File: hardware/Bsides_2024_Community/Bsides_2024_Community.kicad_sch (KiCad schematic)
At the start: 41 parts, among them J1 Conn_02x03_Odd_Even, J2 Battery, J3 Battery, J4 OLED, J5 Conn_01x05, J6 Conn_01x05, P1 USB_C_Plug_USB2.0, Q1 DMG3415U-7, SW1 ON, SW2 RESET, SW3 BOOT, SW4 RESET, SW6 RESET, U1 ESP32-C6-WROOM-1U-N4, U2 AP2112K-3.3

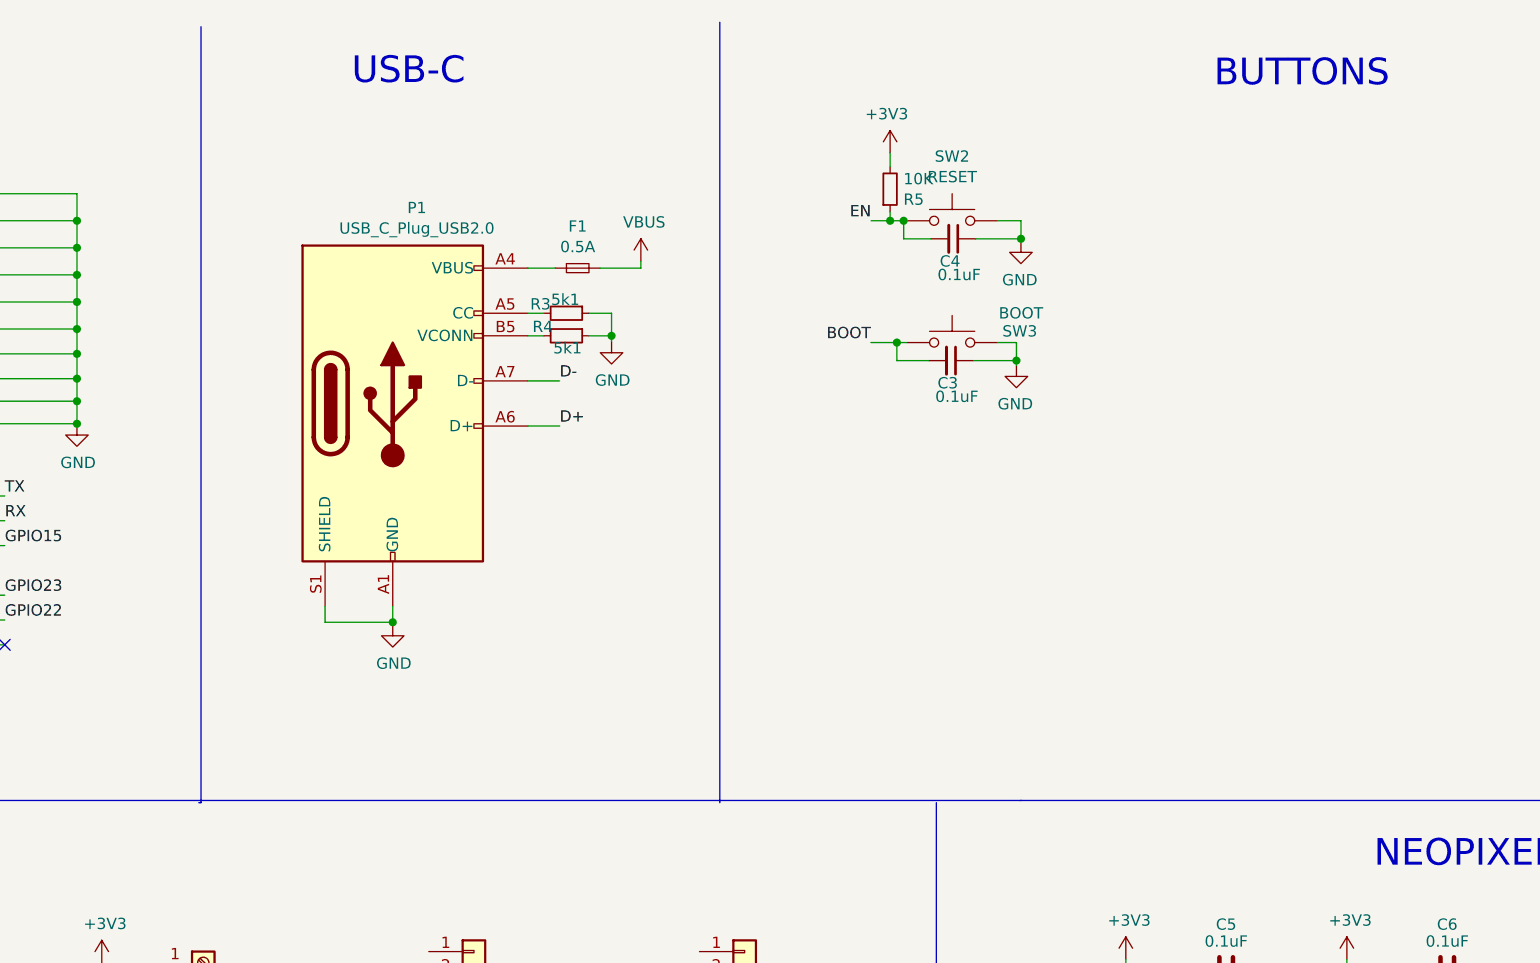
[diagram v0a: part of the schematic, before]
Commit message: feat(Hw): Update PCB
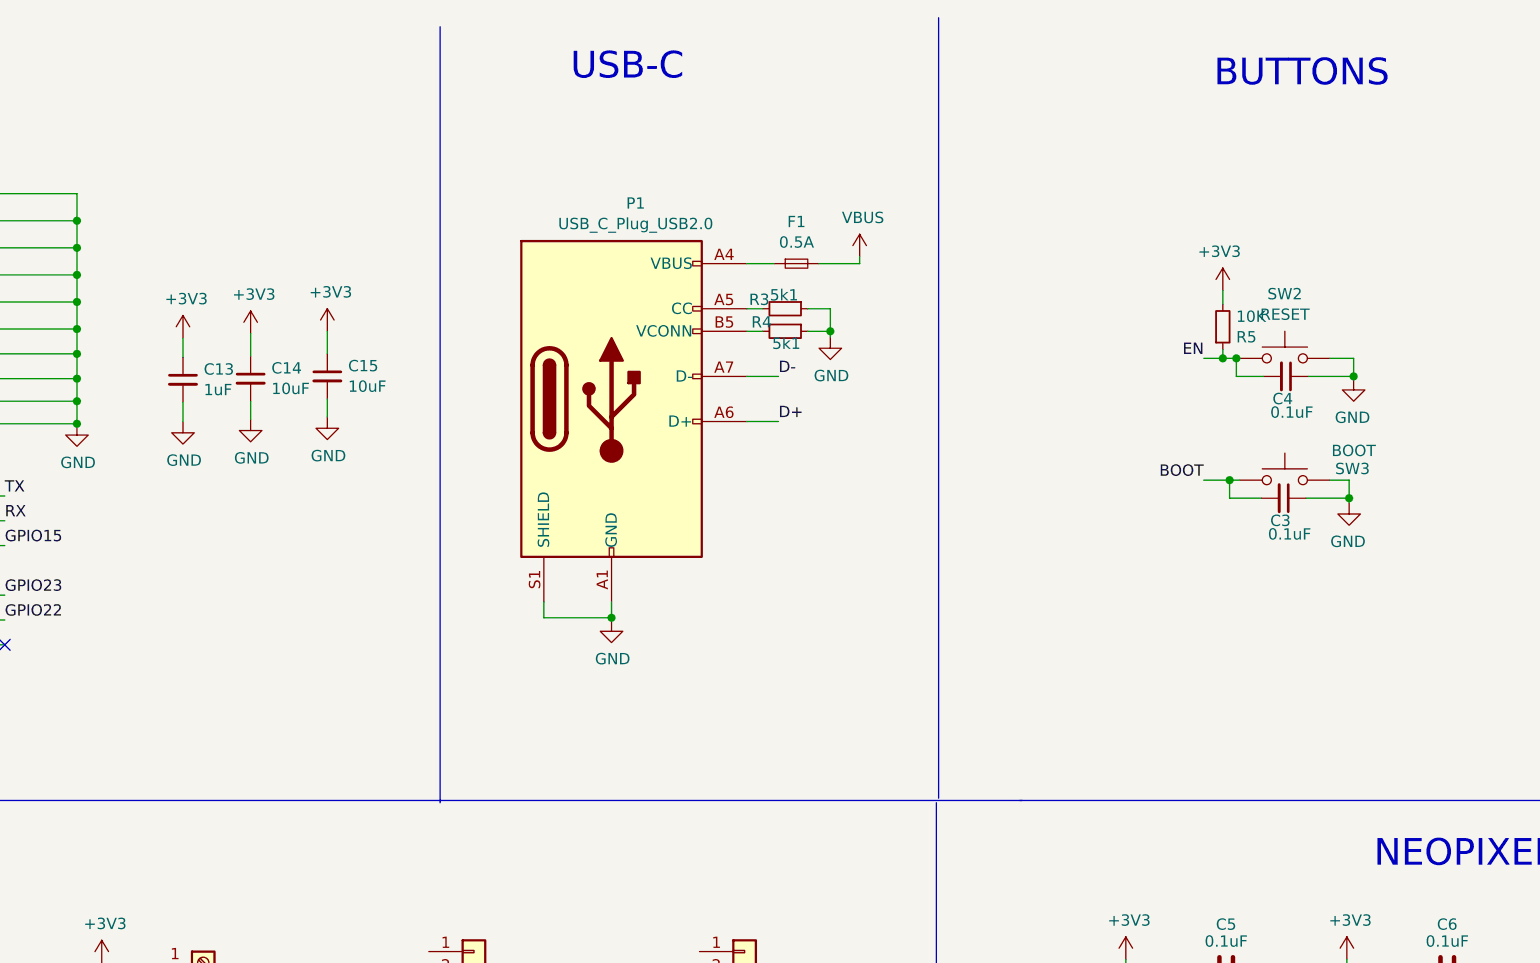
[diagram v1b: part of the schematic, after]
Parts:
- added C13: 1uF, Capacitor_SMD:C_0603_1608Metric, symbol Device:C_Small
- added C14, C15: 10uF, Capacitor_SMD:C_0603_1608Metric, symbol Device:C_Small
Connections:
- net +3V3: now also C13.1, C14.1, C15.1
- net GND: now also C13.2, C14.2, C15.2
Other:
- moved on the sheet: C3, C4, F1, P1, R3, R4, R5, SW2, SW3
